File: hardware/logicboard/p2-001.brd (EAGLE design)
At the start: 72 x 72 mm, 32 parts, among them IC1 5V, IC2 74LS07N, IC3 4066N, IC4 LTC485N, K1 G5V1, T1 2SC1815, U1 DS18B20

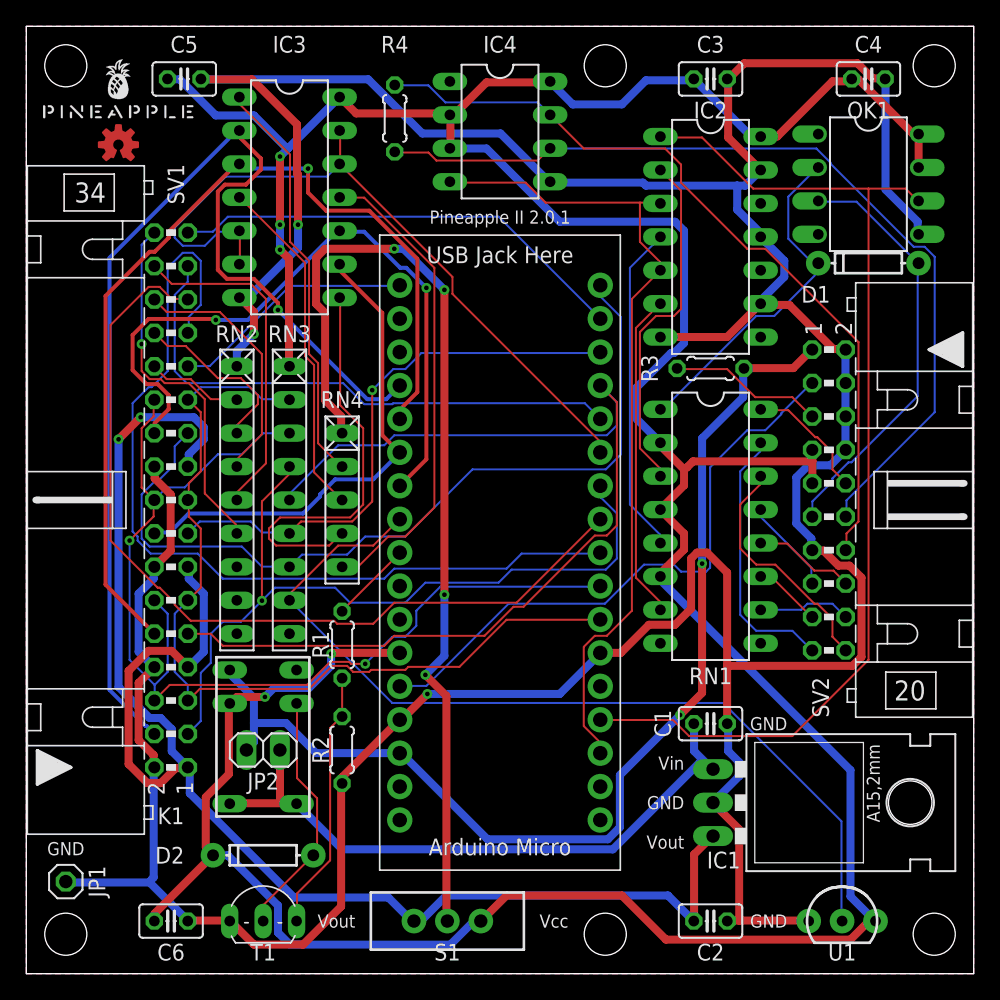
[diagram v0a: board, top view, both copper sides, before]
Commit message: Optimized PCB layout.
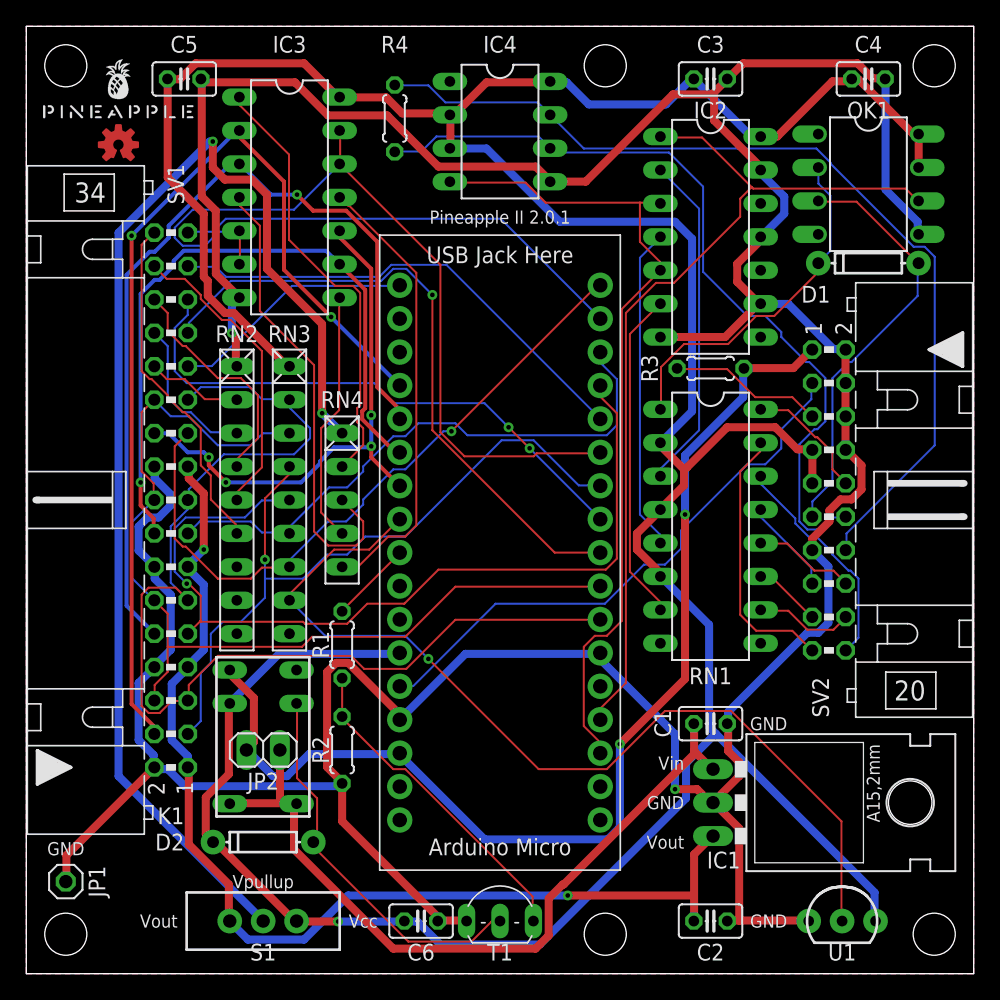
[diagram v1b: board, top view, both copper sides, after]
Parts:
- moved C6 19.0 mm to (30.0, 4.00)
- moved T1 18.0 mm to (36.0, 4.00)
- moved S1 14.0 mm to (18.0, 4.00)
- moved D2 1.00 mm to (18.0, 10.0)
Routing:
- net VOUT: track 118.6 -> 83.2 mm
- net L2: track 67.1 -> 42.9 mm, vias 0 -> 2
- net L1: track 68.4 -> 48.7 mm, vias 0 -> 1
- net VPULLUP: track 74.8 -> 94.3 mm, vias 4 -> 2
- net SDA: track 68.2 -> 84.6 mm
- net A3: track 37.5 -> 52.3 mm, vias 0 -> 1
- net RX: track 80.8 -> 67.7 mm
- net D2: track 79.0 -> 66.4 mm, vias 0 -> 1
- net N$5: track 31.3 -> 19.2 mm
- net D4: track 63.9 -> 51.8 mm, vias 0 -> 1
- net A4: track 53.0 -> 40.9 mm, vias 2 -> 4
- net MTX-: track 60.4 -> 71.6 mm
- net RLYSNK: track 18.9 -> 29.5 mm
- net SCL: track 83.2 -> 72.8 mm, vias 2 -> 0
- net GND: track 320.4 -> 310.8 mm, vias 3 -> 2
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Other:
- board text added: "Vpullup"
